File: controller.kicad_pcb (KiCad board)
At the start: 2 copper layers, 62.4 x 49.5 mm, 38 parts, among them J1 Barrel_Jack_MountingPin, J2 Conn_01x02_Pin, J3 Conn_01x07_Pin, J4 Screw_Terminal_01x06, Q1 IRLTS6342TRPBF, Q2 IRLTS6342TRPBF, Q3 IRLTS6342TRPBF, Q4 IRLTS6342TRPBF, Q5 IRLTS6342TRPBF, SW1 SW_Push, U1 ESP32-C6-DevKitC-1

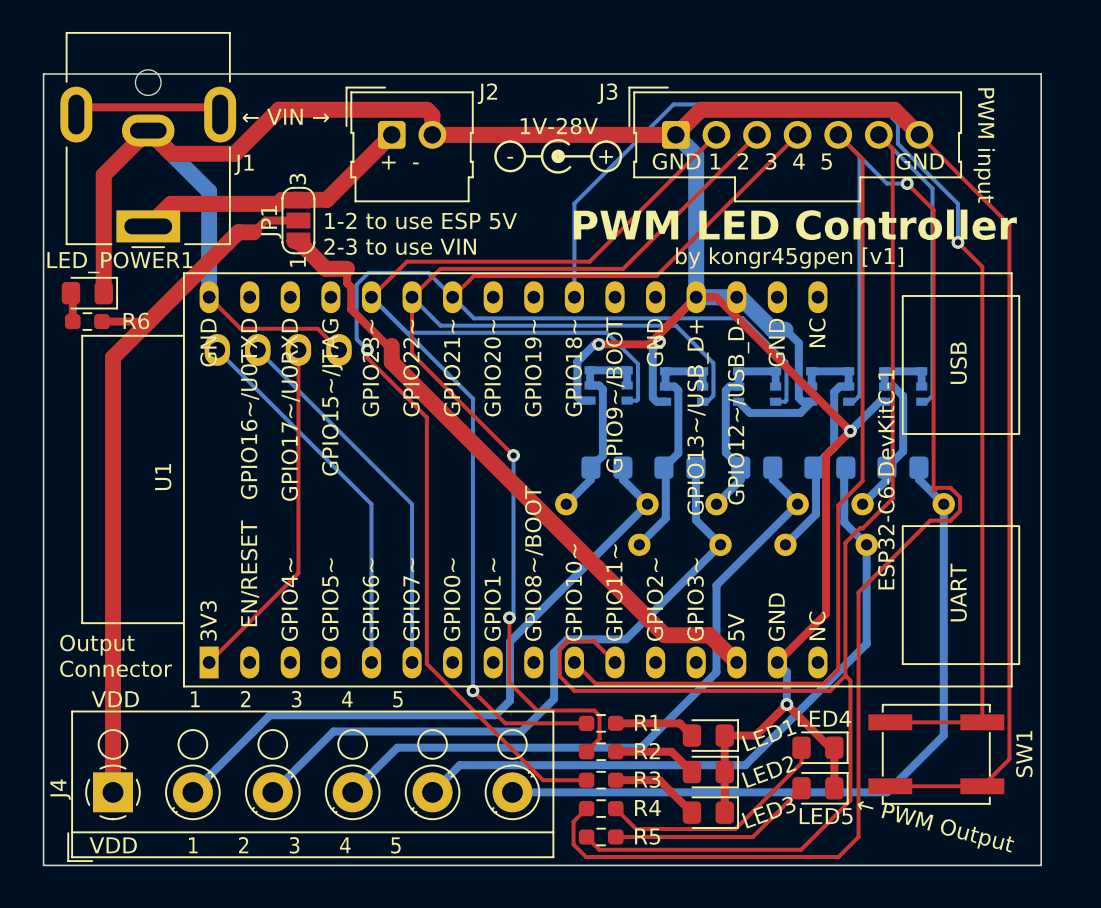
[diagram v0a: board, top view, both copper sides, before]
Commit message: Add figures
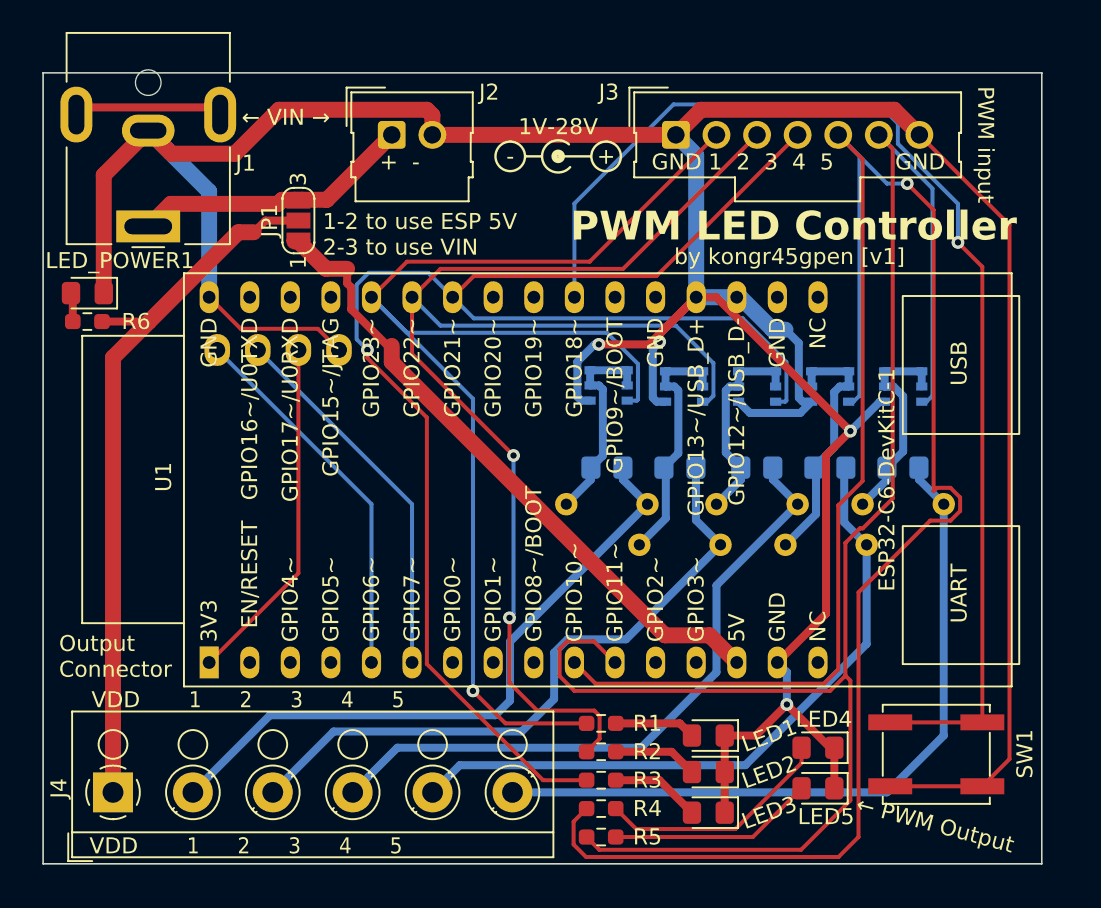
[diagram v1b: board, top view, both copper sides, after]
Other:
- board size 62.4 x 49.5 mm -> 62.5 x 49.5 mm
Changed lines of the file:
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@@
   )
   (gr_rect (start 36.63 26.67) (end 99.06 76.2)
-    (stroke (width 0.1) (type default)) (fill none) (layer "Edge.Cuts"))
+    (stroke (width 0.1) (type default)) (fill none) (layer "Cmts.User"))
+  (gr_line (start 36.6 76.1) (end 36.6 26.6)
+    (stroke (width 0.1) (type default)) (layer "Edge.Cuts"))
+  (gr_line (start 99.1 76.1) (end 36.6 76.1)
+    (stroke (width 0.1) (type default)) (layer "Edge.Cuts"))
+  (gr_line (start 99.1 26.6) (end 99.1 76.1)
+    (stroke (width 0.1) (type default)) (layer "Edge.Cuts"))
+  (gr_line (start 36.6 26.6) (end 99.1 26.6)
+    (stroke (width 0.1) (type default)) (layer "Edge.Cuts"))
   (gr_text "3V3" (at 52.578 45.72 270) (layer "B.SilkS")
     (effects (font (size 1 1) (thickness 0.15)) (justify right mirror))
